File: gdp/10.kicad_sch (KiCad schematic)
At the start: 8 parts, among them IC46 2732, IC47 HM6116, IC50 SCB2675

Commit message: Placing footprints...
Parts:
- R26, R32, R33, R35: footprint Resistor_THT:R_Axial_DIN0207_L6.3mm_D2.5mm_P7.62mm_Horizontal -> Resistor_THT:R_Axial_DIN0207_L6.3mm_D2.5mm_P10.16mm_Horizontal
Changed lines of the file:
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@@
 			)
 		)
-		(property "Footprint" "Resistor_THT:R_Axial_DIN0207_L6.3mm_D2.5mm_P7.62mm_Horizontal"
+		(property "Footprint" "Resistor_THT:R_Axial_DIN0207_L6.3mm_D2.5mm_P10.16mm_Horizontal"
 			(at 234.442 130.81 90)
 			(effects
@@
 			)
 		)
-		(property "Footprint" "Resistor_THT:R_Axial_DIN0207_L6.3mm_D2.5mm_P7.62mm_Horizontal"
+		(property "Footprint" "Resistor_THT:R_Axial_DIN0207_L6.3mm_D2.5mm_P10.16mm_Horizontal"
 			(at 224.917 130.81 90)
 			(effects
@@
 			)
 		)
-		(property "Footprint" "Resistor_THT:R_Axial_DIN0207_L6.3mm_D2.5mm_P7.62mm_Horizontal"
+		(property "Footprint" "Resistor_THT:R_Axial_DIN0207_L6.3mm_D2.5mm_P10.16mm_Horizontal"
 			(at 209.042 45.085 90)
 			(effects
@@
 			)
 		)
-		(property "Footprint" "Resistor_THT:R_Axial_DIN0207_L6.3mm_D2.5mm_P7.62mm_Horizontal"
+		(property "Footprint" "Resistor_THT:R_Axial_DIN0207_L6.3mm_D2.5mm_P10.16mm_Horizontal"
 			(at 185.547 130.81 90)
 			(effects

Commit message: Maps footprints PCB -> sch
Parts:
- R26: footprint Resistor_THT:R_Axial_DIN0207_L6.3mm_D2.5mm_P10.16mm_Horizontal -> GDP:R_XXL
- R33: footprint Resistor_THT:R_Axial_DIN0207_L6.3mm_D2.5mm_P10.16mm_Horizontal -> GDP:R_L
- R35: footprint Resistor_THT:R_Axial_DIN0207_L6.3mm_D2.5mm_P10.16mm_Horizontal -> GDP:R_XL
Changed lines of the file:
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@@
 			)
 		)
-		(property "Footprint" "Resistor_THT:R_Axial_DIN0207_L6.3mm_D2.5mm_P10.16mm_Horizontal"
+		(property "Footprint" "GDP:R_L"
 			(at 234.442 130.81 90)
 			(effects
@@
 			)
 		)
-		(property "Footprint" "Resistor_THT:R_Axial_DIN0207_L6.3mm_D2.5mm_P10.16mm_Horizontal"
+		(property "Footprint" "GDP:R_XXL"
 			(at 209.042 45.085 90)
 			(effects
@@
 			)
 		)
-		(property "Footprint" "Resistor_THT:R_Axial_DIN0207_L6.3mm_D2.5mm_P10.16mm_Horizontal"
+		(property "Footprint" "GDP:R_XL"
 			(at 185.547 130.81 90)
 			(effects

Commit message: Fixes footprint references in sch
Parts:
- R32: footprint Resistor_THT:R_Axial_DIN0207_L6.3mm_D2.5mm_P10.16mm_Horizontal -> GDP:R_L
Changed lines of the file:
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@@
 			)
 		)
-		(property "Footprint" "Resistor_THT:R_Axial_DIN0207_L6.3mm_D2.5mm_P10.16mm_Horizontal"
+		(property "Footprint" "GDP:R_L"
 			(at 224.917 130.81 90)
 			(effects

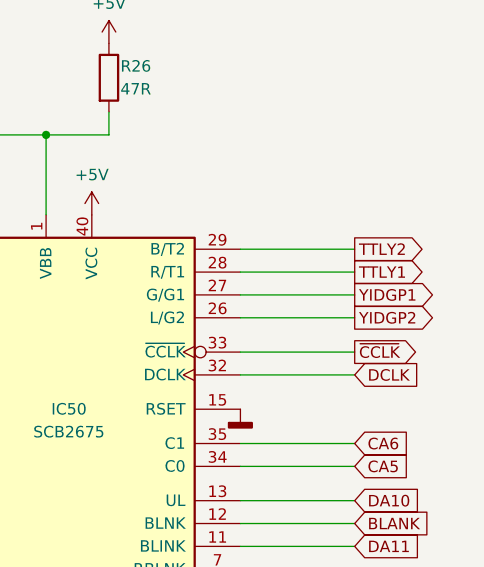
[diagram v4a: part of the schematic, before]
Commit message: Fixes labels
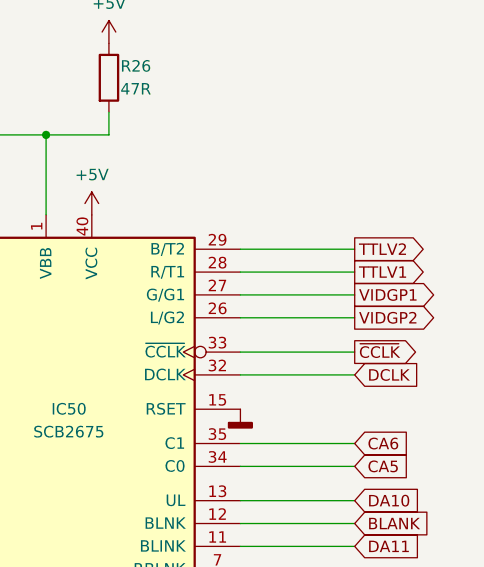
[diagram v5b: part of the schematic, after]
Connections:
- net TTLY1 renamed TTLV1
- net TTLY2 renamed TTLV2
- net YIDGP1 renamed VIDGP1
- net YIDGP2 renamed VIDGP2
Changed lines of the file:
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@@
 		)
 	)
-	(global_label "YIDGP2"
+	(global_label "VIDGP2"
 		(shape output)
 		(at 238.125 71.755 0)
@@
 		)
 	)
-	(global_label "YIDGP1"
+	(global_label "VIDGP1"
 		(shape output)
 		(at 238.125 69.215 0)
@@
 		)
 	)
-	(global_label "TTLY2"
+	(global_label "TTLV2"
 		(shape output)
 		(at 238.125 64.135 0)
@@
 		)
 	)
-	(global_label "TTLY1"
+	(global_label "TTLV1"
 		(shape output)
 		(at 238.125 66.675 0)
